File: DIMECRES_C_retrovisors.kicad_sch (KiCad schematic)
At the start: 92 parts, among them J10 Vbat, J2 DE9_Pins, J3 Conn_01x05_Pin, J4 Motor3, J5 DE9_Pins, J6 Intermitente, J7 Calentador, J8 Motor2, J9 Motor1, Q1 DTC144E, Q2 DTC144E, Q3 DTC144E, SW1 SW_DPDT_G6S, SW10 SW_Push, SW2 SW_Push, SW3 SW_Push, SW4 SW_Push, SW5 SW_Push, SW6 SW_Push, SW7 SW_Push, SW8 FN01B, SW9 FN01B, U1 CH201, U10 LM1117DT-5.0, U2 ADM7160, U3 LM2596S-ADJ, U4 L298N, U5 MCP2551-I-SN, U6 ADA4511-2, U7 PIC18F4480-IP, Y1 Crystal

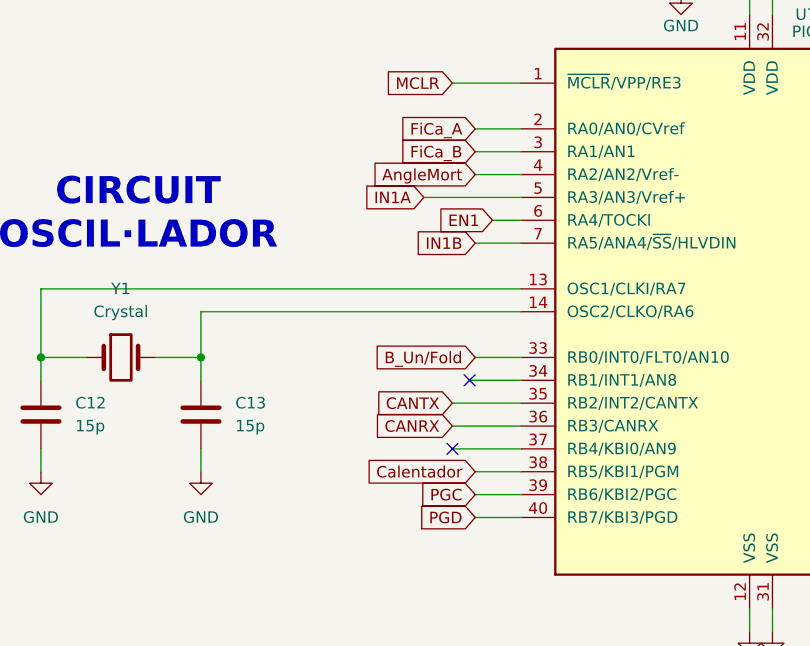
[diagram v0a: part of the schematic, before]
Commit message: correccion errores
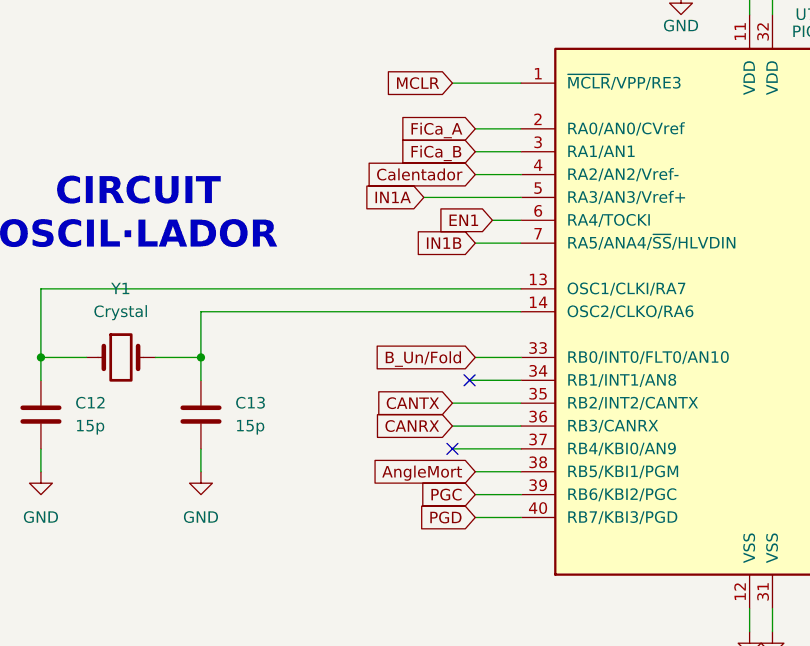
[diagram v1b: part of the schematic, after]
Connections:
- net AngleMort: now also U7.38 (RB5/KBI1/PGM); no longer U7.4 (RA2/AN2/Vref-)
- net Calentador: now also U7.4 (RA2/AN2/Vref-); no longer U7.38 (RB5/KBI1/PGM)
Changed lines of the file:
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@@
 	(global_label "AngleMort"
 		(shape input)
+		(at 79.375 180.975 180)
+		(fields_autoplaced yes)
+		(effects
+			(font
+				(size 1.27 1.27)
+			)
+			(justify right)
+		)
+		(property "Intersheetrefs" "${INTERSHEET_REFS}"
+			(at 67.1371 180.975 0)
+			(effects
+				(font
+					(size 1.27 1.27)
+				)
+				(justify right)
+				(hide yes)
+			)
+		)
+	)
+	(global_label "SENSE_B"
+		(shape input)
+		(at 350.52 170.18 180)
+		(fields_autoplaced yes)
+		(effects
+			(font
+				(size 1.27 1.27)
+			)
+			(justify right)
+		)
+		(property "Intersheetrefs" "${INTERSHEET_REFS}"
+			(at 339.2497 170.18 0)
+			(effects
+				(font
+					(size 1.27 1.27)
+				)
+				(justify right)
+				(hide yes)
+			)
+		)
+	)
+	(global_label "Vbat"
+		(shape input)
+		(at 301.625 212.725 180)
+		(fields_autoplaced yes)
+		(effects
+			(font
+				(size 1.27 1.27)
+			)
+			(justify right)
+		)
+		(property "Intersheetrefs" "${INTERSHEET_REFS}"
+			(at 294.5275 212.725 0)
+			(effects
+				(font
+					(size 1.27 1.27)
+				)
+				(justify right)
+				(hide yes)
+			)
+		)
+	)
+	(global_label "B_Up"
+		(shape input)
+		(at 145.415 150.495 0)
+		(fields_autoplaced yes)
+		(effects
+			(font
+				(size 1.27 1.27)
+			)
+			(justify left)
+		)
+		(property "Intersheetrefs" "${INTERSHEET_REFS}"
+			(at 153.1173 150.495 0)
+			(effects
+				(font
+					(size 1.27 1.27)
+				)
+				(justify left)
+				(hide yes)
+			)
+		)
+	)
+	(global_label "SENSE_A"
+		(shape input)
+		(at 286.385 78.74 270)
+		(fields_autoplaced yes)
+		(effects
+			(font
+				(size 1.27 1.27)
+			)
+			(justify right)
+		)
+		(property "Intersheetrefs" "${INTERSHEET_REFS}"
+			(at 286.385 89.8289 90)
+			(effects
+				(font
+					(size 1.27 1.27)
+				)
+				(justify right)
+				(hide yes)
+			)
+		)
+	)
+	(global_label "Vcc"
+		(shape input)
+		(at 246.38 35.56 90)
+		(fields_autoplaced yes)
+		(effects
+			(font
+				(size 1.27 1.27)
+			)
+			(justify left)
+		)
+		(property "Intersheetrefs" "${INTERSHEET_REFS}"
+			(at 246.38 29.309 90)
+			(effects
+				(font
+					(size 1.27 1.27)
+				)
+				(justify left)
+				(hide yes)
+			)
+		)
+	)
+	(global_label "Act_Rele_M2{slash}M3"
+		(shape input)
+		(at 145.415 160.655 0)
+		(fields_autoplaced yes)
+		(effects
+			(font
+				(size 1.27 1.27)
+			)
+			(justify left)
+		)
+		(property "Intersheetrefs" "${INTERSHEET_REFS}"
+			(at 164.003 160.655 0)
+			(effects
+				(font
+					(size 1.27 1.27)
+				)
+				(justify left)
+				(hide yes)
+			)
+		)
+	)
+	(global_label "B_Un{slash}Fold"
+		(shape input)
+		(at 50.8 71.12 0)
+		(fields_autoplaced yes)
+		(effects
+			(font
+				(size 1.27 1.27)
+			)
+			(justify left)
+		)
+		(property "Intersheetrefs" "${INTERSHEET_REFS}"
+			(at 63.8846 71.12 0)
+			(effects
+				(font
+					(size 1.27 1.27)
+				)
+				(justify left)
+				(hide yes)
+			)
+		)
+	)
+	(global_label "PGD"
+		(shape input)
+		(at 79.375 186.055 180)
+		(fields_autoplaced yes)
+		(effects
+			(font
+				(size 1.27 1.27)
+			)
+			(justify right)
+		)
+		(property "Intersheetrefs" "${INTERSHEET_REFS}"
+			(at 72.5798 186.055 0)
+			(effects
+				(font
+					(size 1.27 1.27)
+				)
+				(justify right)
+				(hide yes)
+			)
+		)
+	)
+	(global_label "Vcc"
+		(shape input)
+		(at 345.44 63.5 180)
+		(fields_autoplaced yes)
+		(effects
+			(font
+				(size 1.27 1.27)
+			)
+			(justify right)
+		)
+		(property "Intersheetrefs" "${INTERSHEET_REFS}"
+			(at 339.189 63.5 0)
+			(effects
+				(font
+					(size 1.27 1.27)
+				)
+				(justify right)
+				(hide yes)
+			)
+		)
+	)
+	(global_label "Calentador"
+		(shape input)
 		(at 79.375 147.955 180)
 		(fields_autoplaced yes)
@@
 		)
 		(property "Intersheetrefs" "${INTERSHEET_REFS}"
-			(at 67.1371 147.955 0)
-			(effects
-				(font
-					(size 1.27 1.27)
-				)
-				(justify right)
-				(hide yes)
-			)
-		)
-	)
-	(global_label "SENSE_B"
-		(shape input)
-		(at 350.52 170.18 180)
-		(fields_autoplaced yes)
-		(effects
-			(font
-				(size 1.27 1.27)
-			)
-			(justify right)
-		)
-		(property "Intersheetrefs" "${INTERSHEET_REFS}"
-			(at 339.2497 170.18 0)
-			(effects
-				(font
-					(size 1.27 1.27)
-				)
-				(justify right)
-				(hide yes)
-			)
-		)
-	)
-	(global_label "Vbat"
-		(shape input)
-		(at 301.625 212.725 180)
-		(fields_autoplaced yes)
-		(effects
-			(font
-				(size 1.27 1.27)
-			)
-			(justify right)
-		)
-		(property "Intersheetrefs" "${INTERSHEET_REFS}"
-			(at 294.5275 212.725 0)
-			(effects
-				(font
-					(size 1.27 1.27)
-				)
-				(justify right)
-				(hide yes)
-			)
-		)
-	)
-	(global_label "B_Up"
-		(shape input)
-		(at 145.415 150.495 0)
-		(fields_autoplaced yes)
-		(effects
-			(font
-				(size 1.27 1.27)
-			)
-			(justify left)
-		)
-		(property "Intersheetrefs" "${INTERSHEET_REFS}"
-			(at 153.1173 150.495 0)
-			(effects
-				(font
-					(size 1.27 1.27)
-				)
-				(justify left)
-				(hide yes)
-			)
-		)
-	)
-	(global_label "SENSE_A"
-		(shape input)
-		(at 286.385 78.74 270)
-		(fields_autoplaced yes)
-		(effects
-			(font
-				(size 1.27 1.27)
-			)
-			(justify right)
-		)
-		(property "Intersheetrefs" "${INTERSHEET_REFS}"
-			(at 286.385 89.8289 90)
-			(effects
-				(font
-					(size 1.27 1.27)
-				)
-				(justify right)
-				(hide yes)
-			)
-		)
-	)
-	(global_label "Vcc"
-		(shape input)
-		(at 246.38 35.56 90)
-		(fields_autoplaced yes)
-		(effects
-			(font
-				(size 1.27 1.27)
-			)
-			(justify left)
-		)
-		(property "Intersheetrefs" "${INTERSHEET_REFS}"
-			(at 246.38 29.309 90)
-			(effects
-				(font
-					(size 1.27 1.27)
-				)
-				(justify left)
-				(hide yes)
-			)
-		)
-	)
-	(global_label "Act_Rele_M2{slash}M3"
-		(shape input)
-		(at 145.415 160.655 0)
-		(fields_autoplaced yes)
-		(effects
-			(font
-				(size 1.27 1.27)
-			)
-			(justify left)
-		)
-		(property "Intersheetrefs" "${INTERSHEET_REFS}"
-			(at 164.003 160.655 0)
-			(effects
-				(font
-					(size 1.27 1.27)
-				)
-				(justify left)
-				(hide yes)
-			)
-		)
-	)
-	(global_label "B_Un{slash}Fold"
-		(shape input)
-		(at 50.8 71.12 0)
-		(fields_autoplaced yes)
-		(effects
-			(font
-				(size 1.27 1.27)
-			)
-			(justify left)
-		)
-		(property "Intersheetrefs" "${INTERSHEET_REFS}"
-			(at 63.8846 71.12 0)
-			(effects
-				(font
-					(size 1.27 1.27)
-				)
-				(justify left)
-				(hide yes)
-			)
-		)
-	)
-	(global_label "PGD"
-		(shape input)
-		(at 79.375 186.055 180)
-		(fields_autoplaced yes)
-		(effects
-			(font
-				(size 1.27 1.27)
-			)
-			(justify right)
-		)
-		(property "Intersheetrefs" "${INTERSHEET_REFS}"
-			(at 72.5798 186.055 0)
-			(effects
-				(font
-					(size 1.27 1.27)
-				)
-				(justify right)
-				(hide yes)
-			)
-		)
-	)
-	(global_label "Vcc"
-		(shape input)
-		(at 345.44 63.5 180)
-		(fields_autoplaced yes)
-		(effects
-			(font
-				(size 1.27 1.27)
-			)
-			(justify right)
-		)
-		(property "Intersheetrefs" "${INTERSHEET_REFS}"
-			(at 339.189 63.5 0)
-			(effects
-				(font
-					(size 1.27 1.27)
-				)
-				(justify right)
-				(hide yes)
-			)
-		)
-	)
-	(global_label "Calentador"
-		(shape input)
-		(at 79.375 180.975 180)
-		(fields_autoplaced yes)
-		(effects
-			(font
-				(size 1.27 1.27)
-			)
-			(justify right)
-		)
-		(property "Intersheetrefs" "${INTERSHEET_REFS}"
-			(at 66.1091 180.975 0)
-			(effects
-				(font
+			(at 66.1091 147.955 0)
+			(effects
+				(font
